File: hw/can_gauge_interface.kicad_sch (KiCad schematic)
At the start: 56 parts, among them U1 MCP2515-I/P, U2 AP64100Q, U3 MCP2561-E-P, U4 25LC160C, U5 PIC16F1459-IP, U6 MCP4912

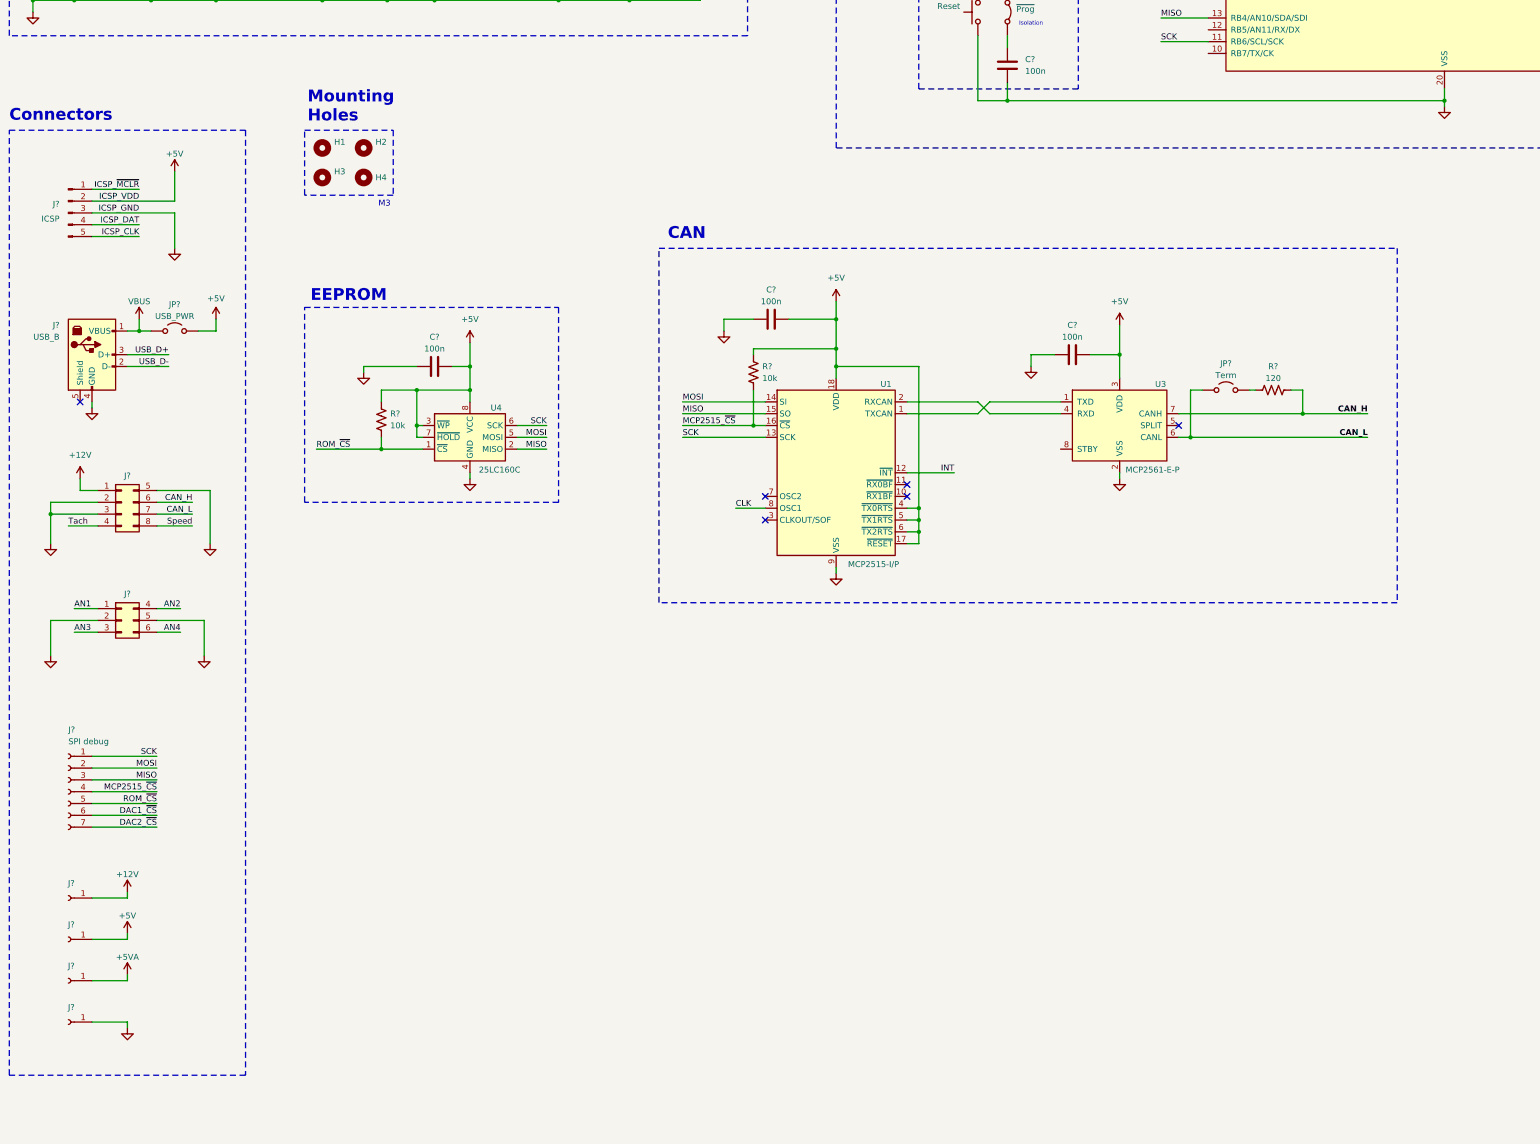
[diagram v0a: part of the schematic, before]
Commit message: hw: 6v6 debug pin
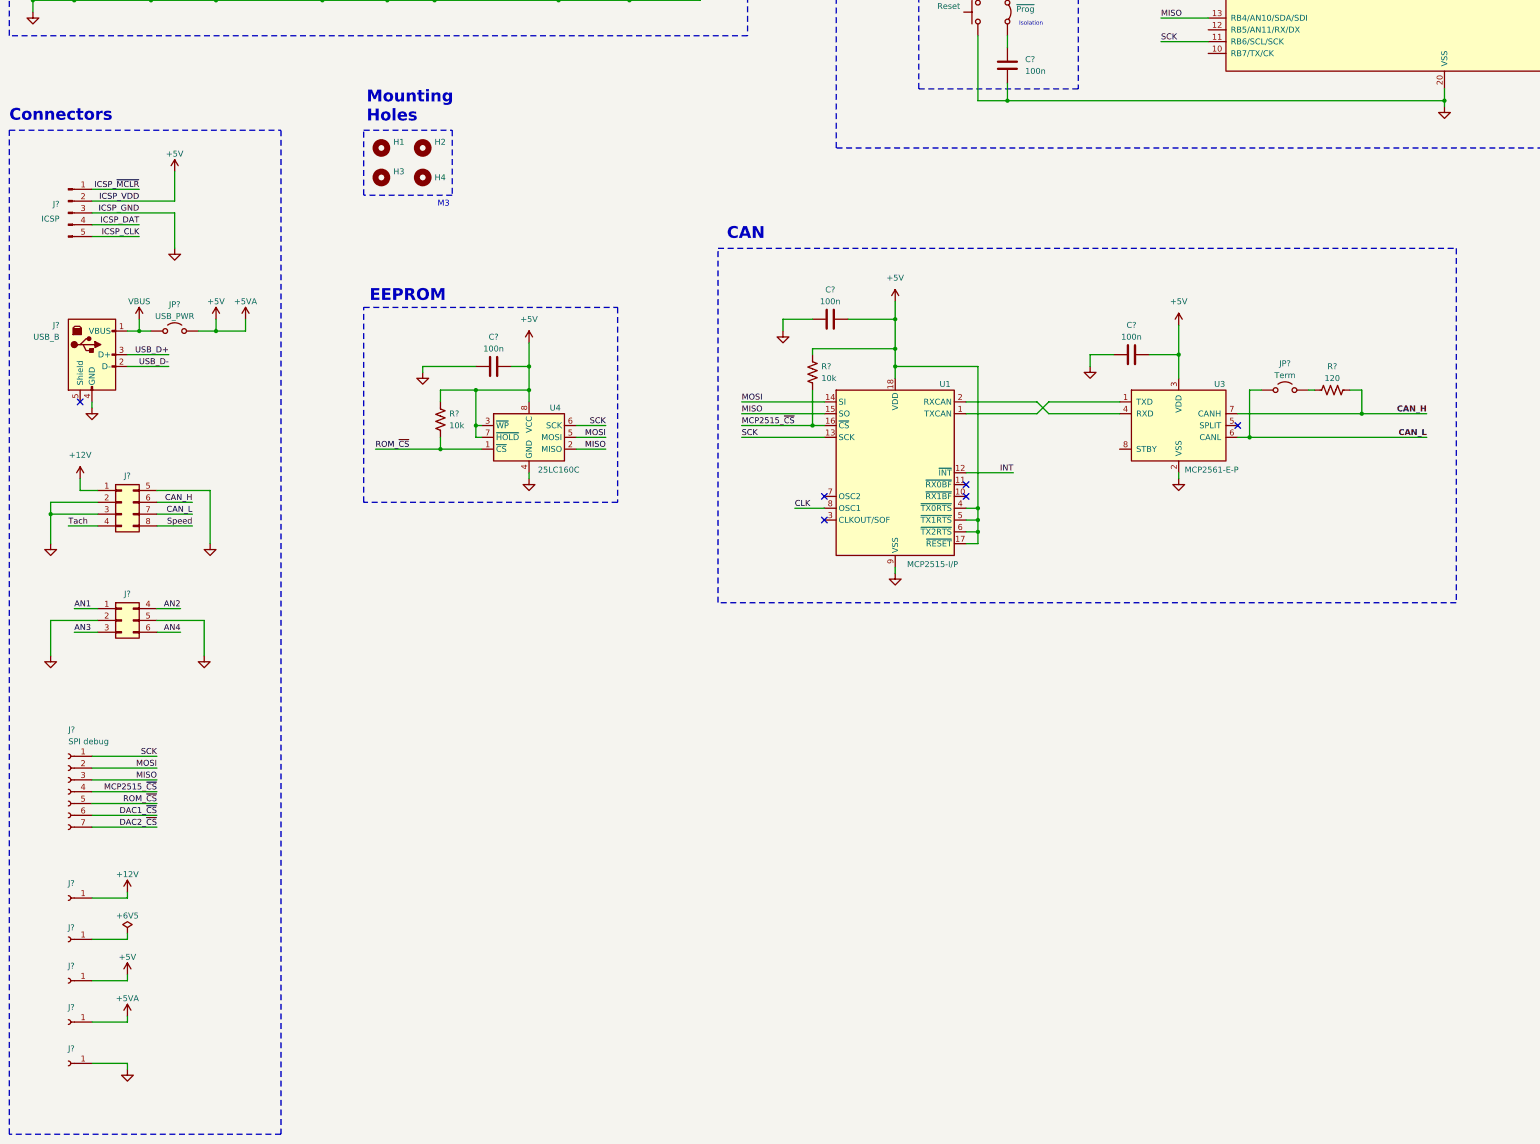
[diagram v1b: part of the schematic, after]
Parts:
- added J?: Conn_01x01_Socket, symbol Connector:Conn_01x01_Socket
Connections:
- net +5VA is gone; now on net +5V: C8.1, C?.1, C?.1, J?.1 (Pin_1), R4.1, R?.1, U6.1 (Vdd), U6.11 (VrefB), U6.13 (VrefA), U6.9 (~{SHDN}), U?.1 (VO), U?.1 (Vdd), U?.11 (VrefB), U?.13 (VrefA), U?.9 (~{SHDN})
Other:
- moved on the sheet: C?, H1, H2, H3, H4, J?, JP?, R?, U1, U3, U4
